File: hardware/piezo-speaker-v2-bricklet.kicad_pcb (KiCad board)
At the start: 2 copper layers, 45 x 55 mm, 38 parts, among them P1 CON-SENSOR2, P2 BOOT, P3 DEBUG, P4 PT-4532PLQ, U1 XMC1XXX24, U2 LD1117, U3 LMR62014X, U4 DRILL, U5 DRILL, U6 DRILL, U7 DRILL

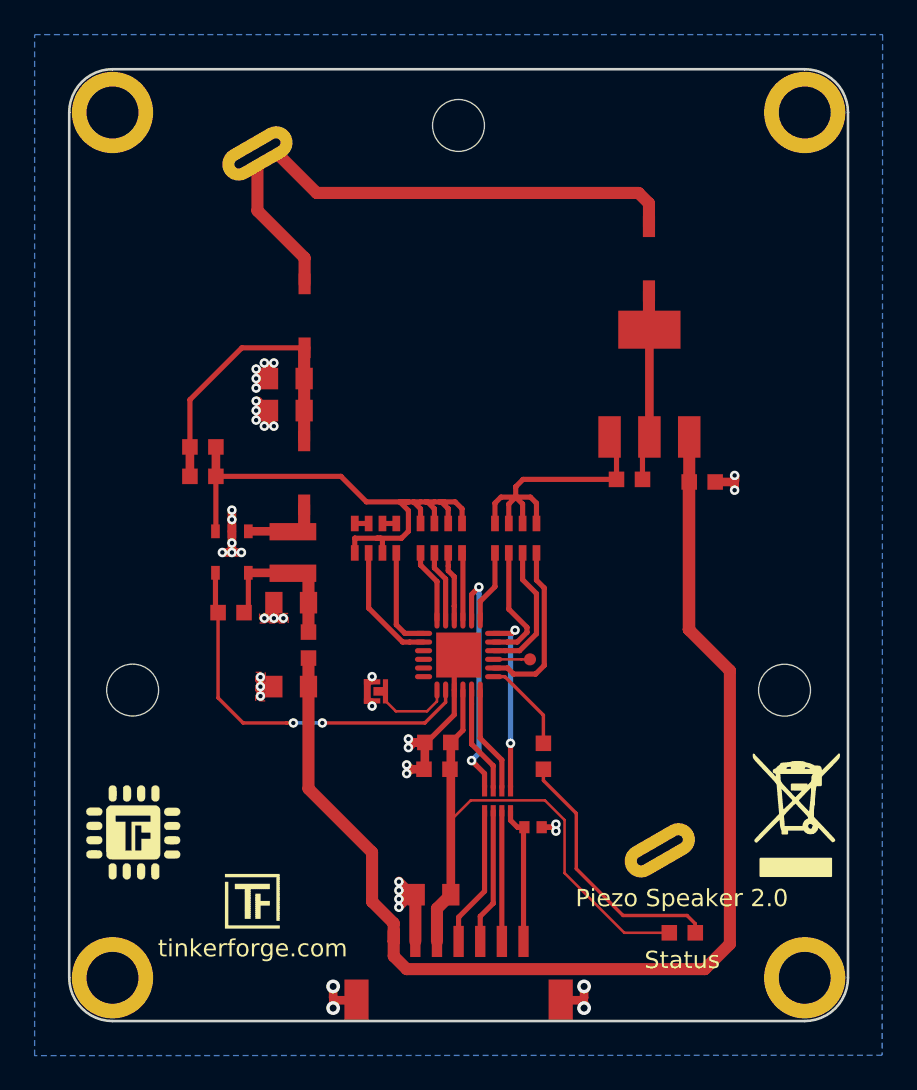
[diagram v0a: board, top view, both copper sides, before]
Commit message: changed the PT footprint, logos, erase and debug pin and first moved the first cap
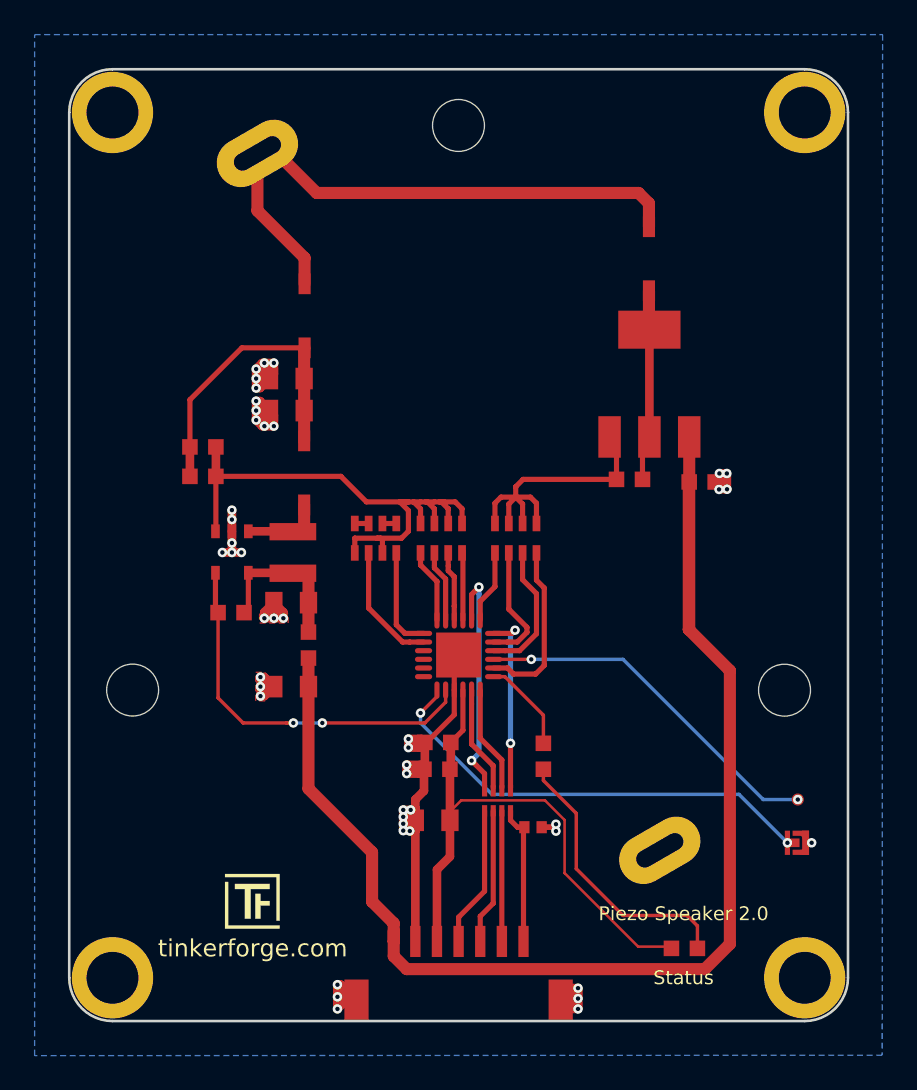
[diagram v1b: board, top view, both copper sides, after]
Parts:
- added VAL: CE_5mm, kicad-libraries:CE_5mm, B.Cu at (162.0, 102.5)
- G***, VAL: moved to B.Cu
- moved VAL 30.8 mm to (148.0, 102.5), turned to 180 degrees
- moved P2 25.9 mm to (174.6, 119.7), turned to 180 degrees
- moved G*** 25.1 mm to (155.0, 102.5), turned to 180 degrees
- moved P3 17.5 mm to (174.6, 117.2)
- moved C2 4.30 mm to (153.5, 118.4)
- moved D1 0.91 mm to (168.1, 125.8)
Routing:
- net GND: track 49.5 -> 82.4 mm, vias 40 -> 45
- net Net-(P2-Pad2): track 5.06 -> 26.8 mm, vias 0 -> 2
- net Net-(P3-Pad1): track 2.10 -> 20.9 mm, vias 0 -> 2
- net Net-(D1-Pad2): track 15.3 -> 16.3 mm
- net 3V3: track 34.9 -> 34.1 mm
